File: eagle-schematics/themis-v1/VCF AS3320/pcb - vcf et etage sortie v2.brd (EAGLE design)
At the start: 78 x 63.8 mm, 42 parts

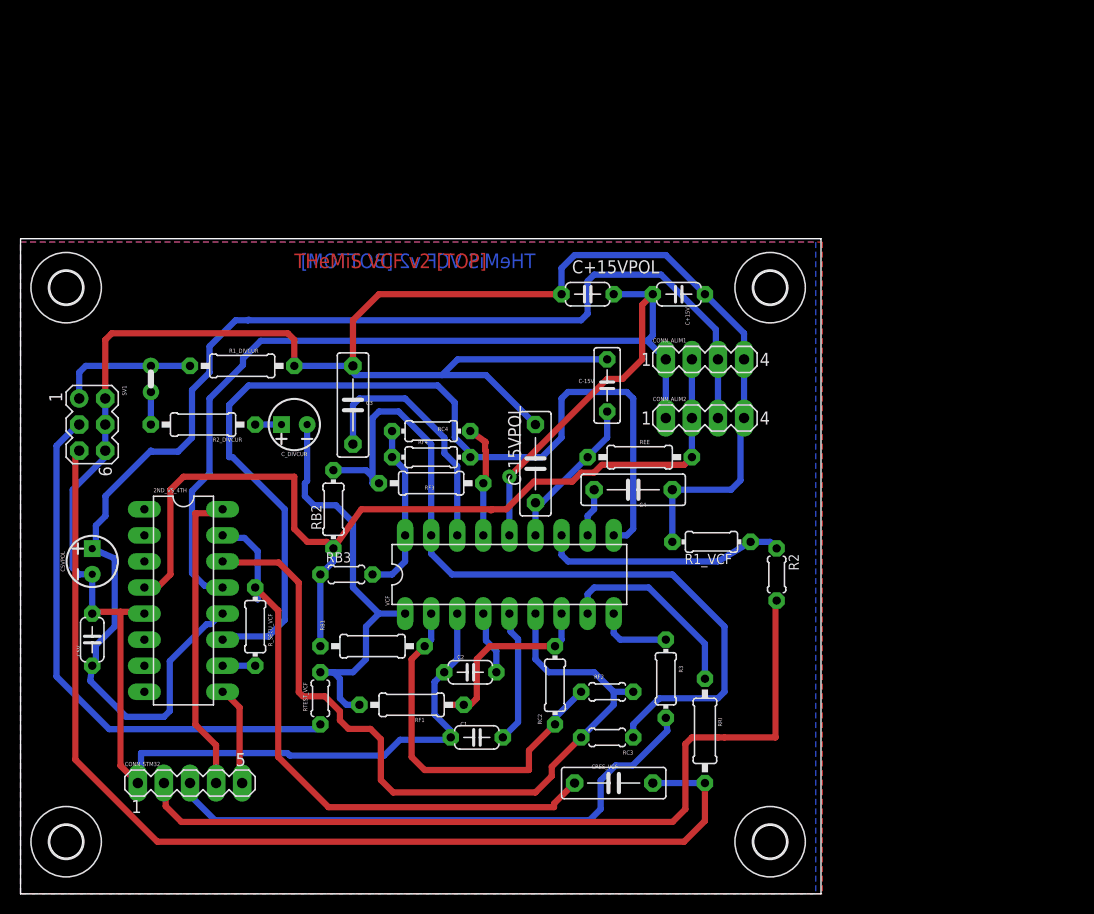
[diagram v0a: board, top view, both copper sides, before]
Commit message: version 1 nouveau pcb vcf
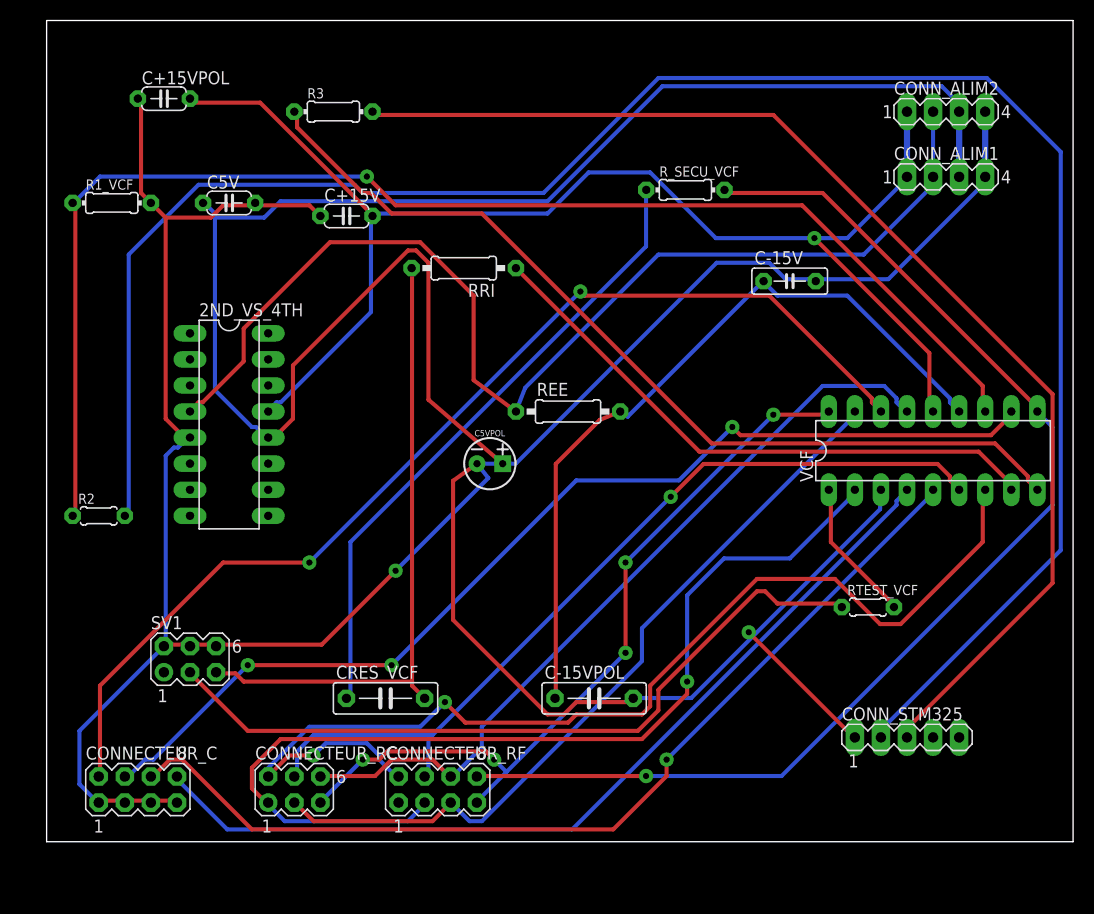
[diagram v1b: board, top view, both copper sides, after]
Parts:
- removed C1, C2: 300p, rcl:C050-024X044
- removed C3, C4: 300p, rcl:C075-032X103
- removed C_DIVCUR: 10uF, SparkFun-Capacitors:CPOL-RADIAL-2.5MM-5MM-KIT
- removed JP_MIXER_OUT: JUMPER_WIRE, 6P1_EVB:JUMPER
- removed R1_DIVCUR, R2_DIVCUR: 470, rcl:0207/10
- removed RB1: 220k, rcl:0207/10
- removed RB2: 220k, rcl:0204/7
- removed RB3: 220k, rcl:0204/5
- removed RC2, RC4: 91k, rcl:0204/7
- removed RC3: 91k, rcl:0204/5
- removed RF1, RF3: 100k, rcl:0207/10
- removed RF2: 100k, rcl:0204/5
- removed RF4: 100k, rcl:0204/7
- removed U$1, U$2, U$3, U$4: (no value), holes:3,2
- added CONNECTEUR_C, CONNECTEUR_RF: (no value), con-lstb:MA04-2
- added CONNECTEUR_RC: (no value), con-lstb:MA03-2
- moved CONN_STM32 70.0 mm to (83.8, 10.2)
- moved R1_VCF 67.1 mm to (6.35, 62.2), turned to 0 degrees
- moved R2 66.3 mm to (5.08, 31.8), turned to 0 degrees
- moved R3 64.0 mm to (27.9, 71.1), turned to 0 degrees
- moved R_SECU_VCF 59.7 mm to (62.2, 63.5), turned to 0 degrees
- moved RTEST_VCF 54.1 mm to (80.0, 22.9), turned to 0 degrees
- moved RRI 50.8 mm to (40.6, 55.9), turned to 180 degrees
- moved C+15VPOL 45.5 mm to (11.4, 72.4)
- moved C5V 44.6 mm to (17.8, 62.2), turned to 0 degrees
- moved VCF 43.0 mm to (86.4, 38.1)
- moved C5VPOL 39.9 mm to (43.2, 36.8), turned to 0 degrees
- moved CONN_ALIM2 38.0 mm to (87.6, 71.1)
- moved C+15V 33.3 mm to (29.2, 61.0), turned to 0 degrees
- moved CONN_ALIM1 29.5 mm to (87.6, 64.8)
- moved SV1 24.8 mm to (14.0, 17.8), turned to 0 degrees
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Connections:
- removed net N$17: C3.2, VCF.16
- removed net N$18: C2.2, VCF.4
- removed net N$24: C4.2, VCF.11
- removed net N$57: RC2.2, RF1.1, VCF.7
- removed net N$62: RB1.2, RC2.1, RF2.1, VCF.2
- removed net N$65: 2ND_VS_4TH.14, RC3.2, RF2.2, VCF.6
- removed net N$72: RB2.2, RC3.1, RF3.1, VCF.17
- removed net N$73: 2ND_VS_4TH.10, R_SECU_VCF.2
- removed net N$75: C_DIVCUR.1, R2_DIVCUR.1
- removed net N$79: JP_MIXER_OUT.2, R2_DIVCUR.2
- removed net N$82: RC4.2, RF3.2, VCF.15
- removed net N$83: RB3.2, RC4.1, RF4.1, VCF.18
- new net N$1: CONNECTEUR_RF.1
- new net N$10: CONNECTEUR_RC.6, CONNECTEUR_RF.6, VCF.15
- new net N$11: CONNECTEUR_RC.5, CONNECTEUR_RF.7, VCF.18
- new net N$2: CONNECTEUR_RC.2, CONNECTEUR_RF.2, VCF.7
- new net N$3: CONNECTEUR_C.4, VCF.11
- new net N$4: CONNECTEUR_C.2, VCF.16
- new net N$6: CONNECTEUR_C.6, VCF.5
- new net N$7: CONNECTEUR_RC.1, CONNECTEUR_RF.3, VCF.2
- new net N$8: CONNECTEUR_RC.4, CONNECTEUR_RF.4, VCF.6
- new net N$9: CONNECTEUR_RC.3, CONNECTEUR_RF.5, VCF.17
- net -15V: no longer RB1.1, RB2.1, RB3.1
- net AGND: now also CONNECTEUR_C.1, CONNECTEUR_C.3, CONNECTEUR_C.5, CONNECTEUR_C.7; no longer C1.1, C2.1, C3.1, C4.1, R1_DIVCUR.2
- net IN_2NDORDER: no longer 2ND_VS_4TH.16
- net IN_4THORDER: no longer 2ND_VS_4TH.9
- net I_IN: no longer JP_MIXER_OUT.1, R1_DIVCUR.1
- net N$5: now also CONNECTEUR_C.8, VCF.4; no longer C1.2, VCF.5
- net N$58: no longer 2ND_VS_4TH.15
- net N$69: now also CONNECTEUR_RF.8, R_SECU_VCF.2; no longer 2ND_VS_4TH.11, RF4.2
- net VCF_IN: no longer C_DIVCUR.2, RF1.2
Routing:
- net CV_CUTOFF: track 82.9 -> 191.5 mm
- net N$37: track 23.9 -> 131.5 mm, vias 0 -> 1
- net N$2: track 0.00 -> 106.8 mm, vias 0 -> 2
- net N$4: track 0.00 -> 106.0 mm, vias 0 -> 2
- net N$3: track 0.00 -> 102.0 mm, vias 0 -> 3
- net N$7: track 0.00 -> 96.9 mm, vias 0 -> 1
- net N$6: track 0.00 -> 94.5 mm, vias 0 -> 1
- net N$8: track 0.00 -> 84.6 mm, vias 0 -> 1
- net N$87: track 7.25 -> 88.6 mm
- net N$72: track 79.5 -> 0.00 mm
- net N$65: track 77.2 -> 0.00 mm
- net N$10: track 0.00 -> 76.7 mm
- net N$11: track 0.00 -> 76.4 mm, vias 0 -> 5
- net N$9: track 0.00 -> 75.5 mm
- net N$5: track 13.0 -> 87.3 mm
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- removed copper zone on layer 1, net AGND
- removed copper zone on layer 16, net AGND
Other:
- board size 78 x 63.8 mm -> 100 x 80 mm
- board text removed: "THeMiS VCF v2 [BOTTOM]"
- board text removed: "THeMiS VCF v2 [TOP]"
